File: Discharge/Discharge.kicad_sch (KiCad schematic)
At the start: 12 parts, among them K2 Relay_SPDT, Q1 2N7002-TP, U1 NE555DR, U2 CPC1017NTR

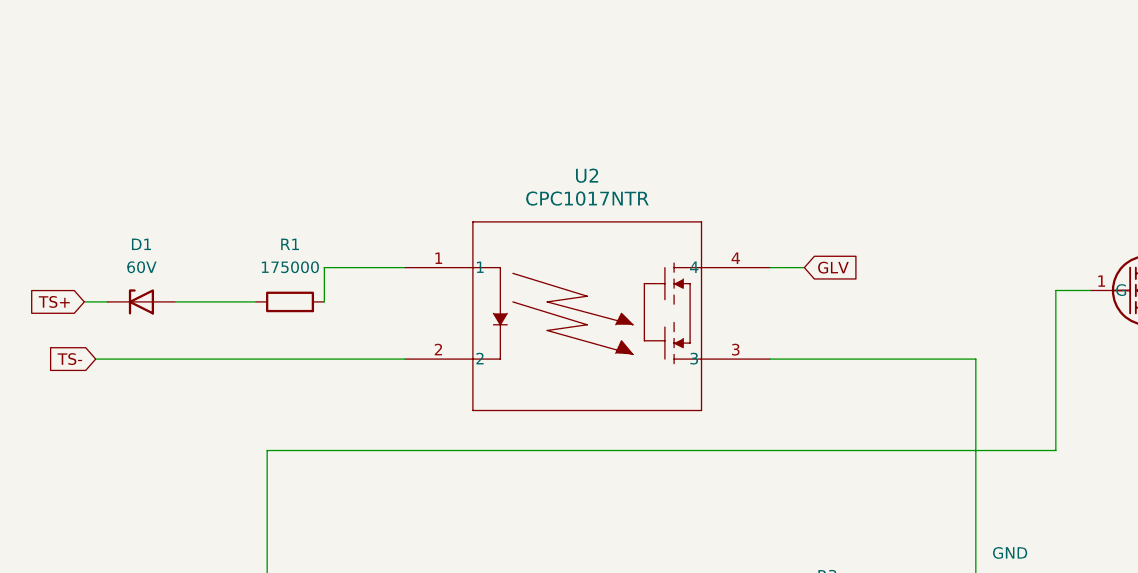
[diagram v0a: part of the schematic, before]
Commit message: opto
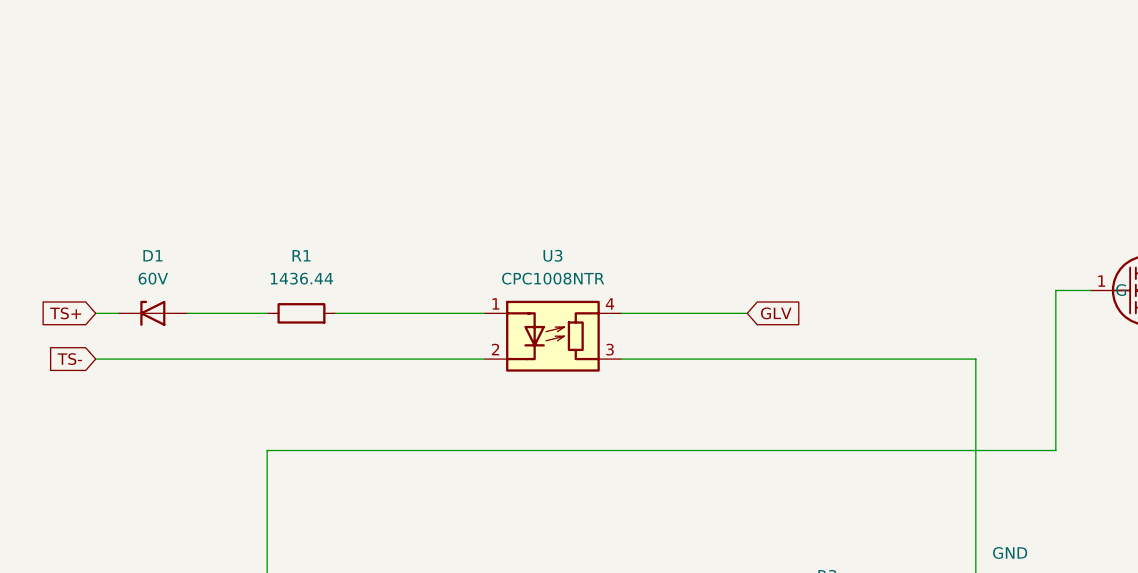
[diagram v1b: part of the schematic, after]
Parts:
- removed U2: CPC1017NTR, CPC1008N_IXY, symbol New_Library:CPC1017NTR
- added U3: CPC1008NTR, Library:CPC1008N_IXY, symbol Isolator:NSL-32
- R1: value 175000 -> 1436.44
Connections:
- net GLV: now also U3.4 (R)
- net TS-: now also U3.2 (K)
- net at R1.2: now also U3.1 (A)
- net at C2.2, R2.2, R3.2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: now also U3.3 (R)
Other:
- moved on the sheet: D1, R1
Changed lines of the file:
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@@
-	(wire
-		(pts
-			(xy 119.38 95.25) (xy 142.24 95.25)
-		)
-		(stroke
-			(width 0)
-			(type default)
-		)
-	)
 	(wire
 		(pts
@@
 	(wire
 		(pts
+			(xy 102.87 90.17) (xy 116.84 90.17)
+		)
+		(stroke
+			(width 0)
+			(type default)
+		)
+	)
+	(wire
+		(pts
 			(xy 140.97 143.51) (xy 142.24 143.51)
 		)
@@
 	(wire
 		(pts
-			(xy 69.85 85.09) (xy 78.74 85.09)
-		)
-		(stroke
-			(width 0)
-			(type default)
-		)
-	)
-	(wire
-		(pts
-			(xy 43.18 88.9) (xy 45.72 88.9)
+			(xy 44.45 90.17) (xy 46.99 90.17)
 		)
 		(stroke
@@
 	(wire
 		(pts
-			(xy 53.34 88.9) (xy 62.23 88.9)
+			(xy 54.61 90.17) (xy 63.5 90.17)
 		)
 		(stroke
@@
 	(wire
 		(pts
-			(xy 69.85 88.9) (xy 69.85 85.09)
-		)
-		(stroke
-			(width 0)
-			(type default)
-		)
-	)
-	(wire
-		(pts
 			(xy 241.3 73.66) (xy 241.3 76.2)
 		)
@@
 	(wire
 		(pts
-			(xy 44.45 95.25) (xy 78.74 95.25)
-		)
-		(stroke
-			(width 0)
-			(type default)
-		)
-	)
-	(wire
-		(pts
 			(xy 68.58 149.86) (xy 69.85 149.86)
 		)
@@
 	(wire
 		(pts
+			(xy 102.87 95.25) (xy 142.24 95.25)
+		)
+		(stroke
+			(width 0)
+			(type default)
+		)
+	)
+	(wire
+		(pts
 			(xy 146.05 134.62) (xy 149.86 134.62)
 		)
@@
 	(wire
 		(pts
-			(xy 119.38 85.09) (xy 123.19 85.09)
-		)
-		(stroke
-			(width 0)
-			(type default)
-		)
-	)
-	(wire
-		(pts
 			(xy 149.86 162.56) (xy 68.58 162.56)
 		)
@@
 		(pts
 			(xy 73.66 148.59) (xy 72.39 148.59)
+		)
+		(stroke
+			(width 0)
+			(type default)
+		)
+	)
+	(wire
+		(pts
+			(xy 44.45 95.25) (xy 87.63 95.25)
+		)
+		(stroke
+			(width 0)
+			(type default)
+		)
+	)
+	(wire
+		(pts
+			(xy 71.12 90.17) (xy 87.63 90.17)
 		)
 		(stroke
@@
 	(global_label "TS+"
 		(shape input)
-		(at 43.18 88.9 180)
+		(at 44.45 90.17 180)
 		(fields_autoplaced yes)
 		(effects
@@
 		)
 		(property "Intersheetrefs" "${INTERSHEET_REFS}"
-			(at 36.4453 88.9 0)
+			(at 37.7153 90.17 0)
 			(effects
 				(font
@@
 	(global_label "GLV"
 		(shape input)
-		(at 123.19 85.09 0)
+		(at 116.84 90.17 0)
 		(fields_autoplaced yes)
 		(effects
@@
 		)
 		(property "Intersheetrefs" "${INTERSHEET_REFS}"
-			(at 129.5619 85.09 0)
+			(at 123.2119 90.17 0)
 			(effects
 				(font
@@
 	(symbol
 		(lib_id "Device:R")
-		(at 66.04 88.9 90)
+		(at 67.31 90.17 90)
 		(unit 1)
 		(exclude_from_sim no)
@@
 		(fields_autoplaced yes)
 		(property "Reference" "R1"
-			(at 66.04 82.55 90)
-			(effects
-				(font
-					(size 1.27 1.27)
-				)
-			)
-		)
-		(property "Value" "175000"
-			(at 66.04 85.09 90)
+			(at 67.31 83.82 90)
+			(effects
+				(font
+					(size 1.27 1.27)
+				)
+			)
+		)
+		(property "Value" "1436.44"
+			(at 67.31 86.36 90)
 			(effects
 				(font
@@
 		)
 		(property "Footprint" ""
-			(at 66.04 90.678 90)
+			(at 67.31 91.948 90)
 			(effects
 				(font
@@
 		)
 		(property "Datasheet" "~"
-			(at 66.04 88.9 0)
+			(at 67.31 90.17 0)
 			(effects
 				(font
@@
 		)
 		(property "Description" ""
-			(at 66.04 88.9 0)
+			(at 67.31 90.17 0)
 			(effects
 				(font
@@
 	)
 	(symbol
-		(lib_id "New_Library:CPC1017NTR")
-		(at 78.74 85.09 0)
-		(unit 1)
-		(exclude_from_sim no)
-		(in_bom yes)
-		(on_board yes)
-		(dnp no)
-		(fields_autoplaced yes)
-		(property "Reference" "U2"
-			(at 99.06 74.93 0)
-			(effects
-				(font
-					(size 1.524 1.524)
-				)
-			)
-		)
-		(property "Value" "CPC1017NTR"
-			(at 99.06 77.47 0)
-			(effects
-				(font
-					(size 1.524 1.524)
-				)
-			)
-		)
-		(property "Footprint" "CPC1008N_IXY"
-			(at 78.74 85.09 0)
-			(effects
-				(font
-					(size 1.27 1.27)
-					(italic yes)
-				)
-				(hide yes)
-			)
-		)
-		(property "Datasheet" "CPC1017NTR"
-			(at 78.74 85.09 0)
-			(effects
-				(font
-					(size 1.27 1.27)
-					(italic yes)
-				)
-				(hide yes)
-			)
-		)
-		(property "Description" ""
-			(at 78.74 85.09 0)
-			(effects
-				(font
-					(size 1.27 1.27)
-				)
-				(hide yes)
-			)
-		)
-		(pin "4"
-		)
-		(pin "1"
-		)
-		(pin "3"
-		)
-		(pin "2"
-		)
-		(instances
-			(project "Discharge"
-				(path "/dc0f9272-e025-432b-a444-53b3815238aa"
-					(reference "U2")
-					(unit 1)
-				)
-			)
-		)
-	)
-	(symbol
 		(lib_name "GND_4")
 		(lib_id "power:GND")
@@
 	(symbol
 		(lib_id "Device:D_Zener")
-		(at 49.53 88.9 0)
+		(at 50.8 90.17 0)
 		(unit 1)
 		(exclude_from_sim no)
@@
 		(fields_autoplaced yes)
 		(property "Reference" "D1"
-			(at 49.53 82.55 0)
+			(at 50.8 83.82 0)
 			(effects
 				(font
@@
 		)
 		(property "Value" "60V"
-			(at 49.53 85.09 0)
+			(at 50.8 86.36 0)
 			(effects
 				(font
@@
 		)
 		(property "Footprint" ""
-			(at 49.53 88.9 0)
+			(at 50.8 90.17 0)
 			(effects
 				(font
@@
 		)
 		(property "Datasheet" "~"
-			(at 49.53 88.9 0)
+			(at 50.8 90.17 0)
 			(effects
 				(font
@@
 		)
 		(property "Description" ""
-			(at 49.53 88.9 0)
+			(at 50.8 90.17 0)
 			(effects
 				(font
@@
 					(unit 1)
 				)
+			)
+		)
+	)
+	(symbol
+		(lib_id "Isolator:NSL-32")
+		(at 95.25 92.71 0)
+		(unit 1)
+		(exclude_from_sim no)
+		(in_bom yes)
+		(on_board yes)
+		(dnp no)
+		(fields_autoplaced yes)
+		(property "Reference" "U3"
+			(at 95.25 83.82 0)
+			(effects
+				(font
+					(size 1.27 1.27)
+				)
+			)
+		)
+		(property "Value" "CPC1008NTR"
+			(at 95.25 86.36 0)
+			(effects
+				(font
+					(size 1.27 1.27)
+				)
+			)
+		)
+		(property "Footprint" "Library:CPC1008N_IXY"
+			(at 95.25 100.33 0)
+			(effects
+				(font
+					(size 1.27 1.27)
+				)
+				(hide yes)
+			)
+		)
+		(property "Datasheet" "http://lunainc.com/wp-content/uploads/2016/06/NSL-32.pdf"
+			(at 96.52 92.71 0)
+			(effects
+				(font
+					(size 1.27 1.27)
+				)
+				(hide yes)
+			)
+		)
+		(property "Description" "Optocoupler, LED Input, Photocell Output"
+			(at 95.25 92.71 0)
+			(effects
+				(font
+					(size 1.27 1.27)
+				)
+				(hide yes)
+			)
+		)
+		(pin "1"
+		)
+		(pin "4"
+		)
+		(pin "2"
+		)
+		(pin "3"
+		)
+		(instances
+			(project ""
+				(path "/dc0f9272-e025-432b-a444-53b3815238aa"
+					(reference "U3")
+					(unit 1)
+				)
